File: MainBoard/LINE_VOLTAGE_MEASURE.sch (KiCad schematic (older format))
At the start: 18 parts

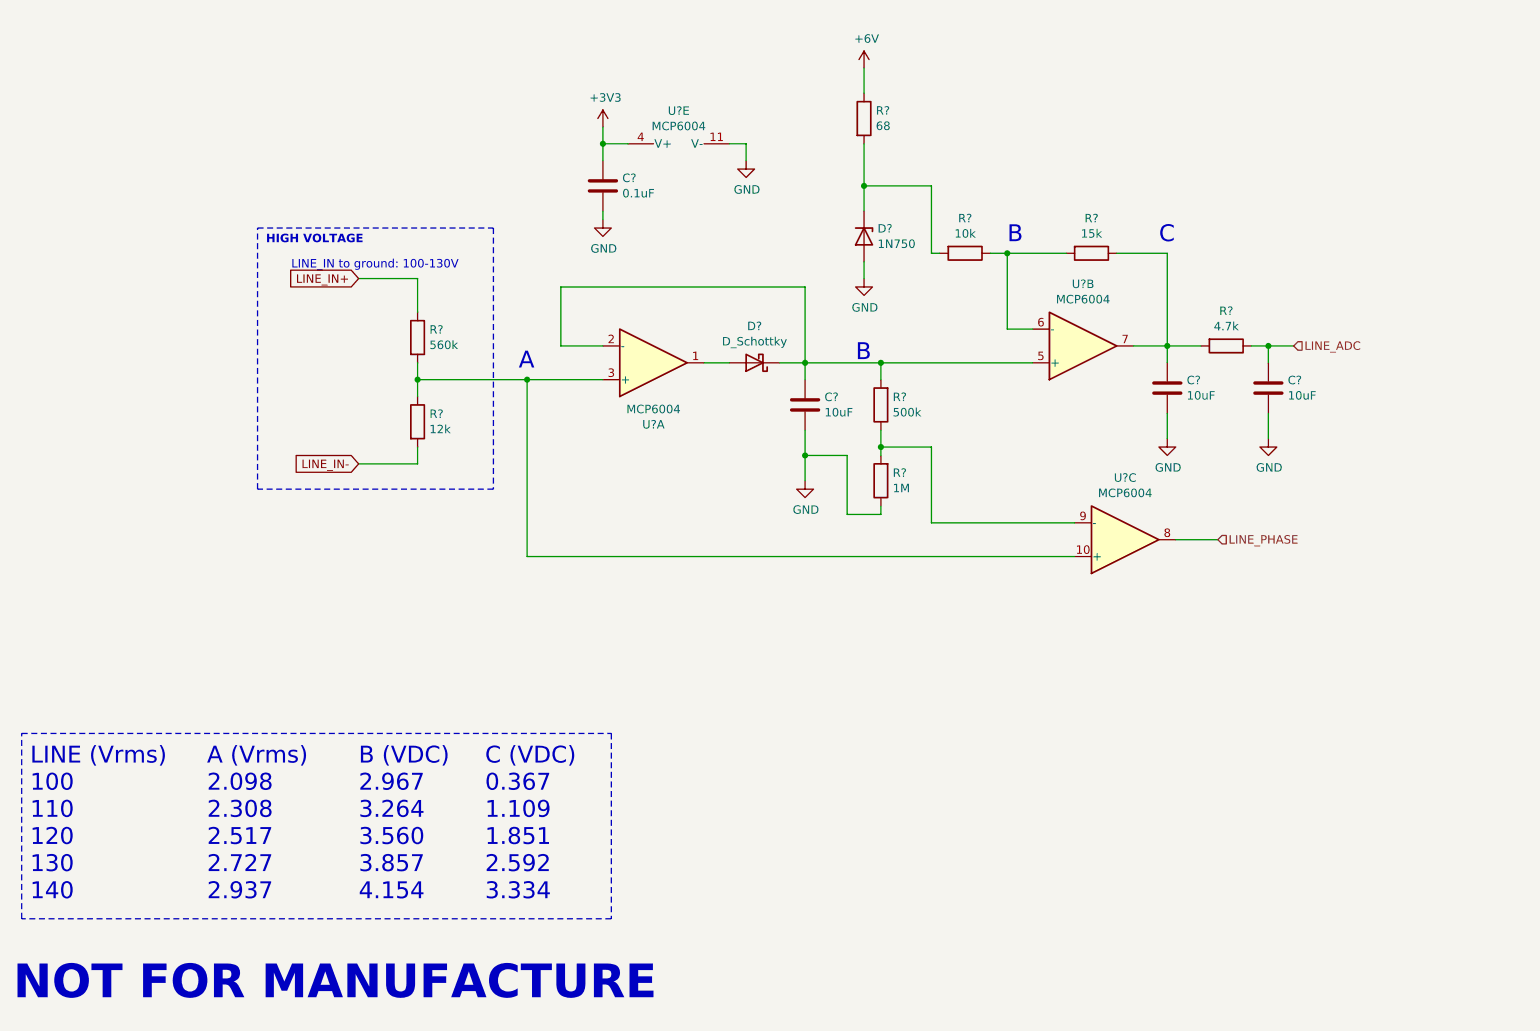
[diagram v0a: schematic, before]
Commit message: Layout Main Board
Layout main PCB
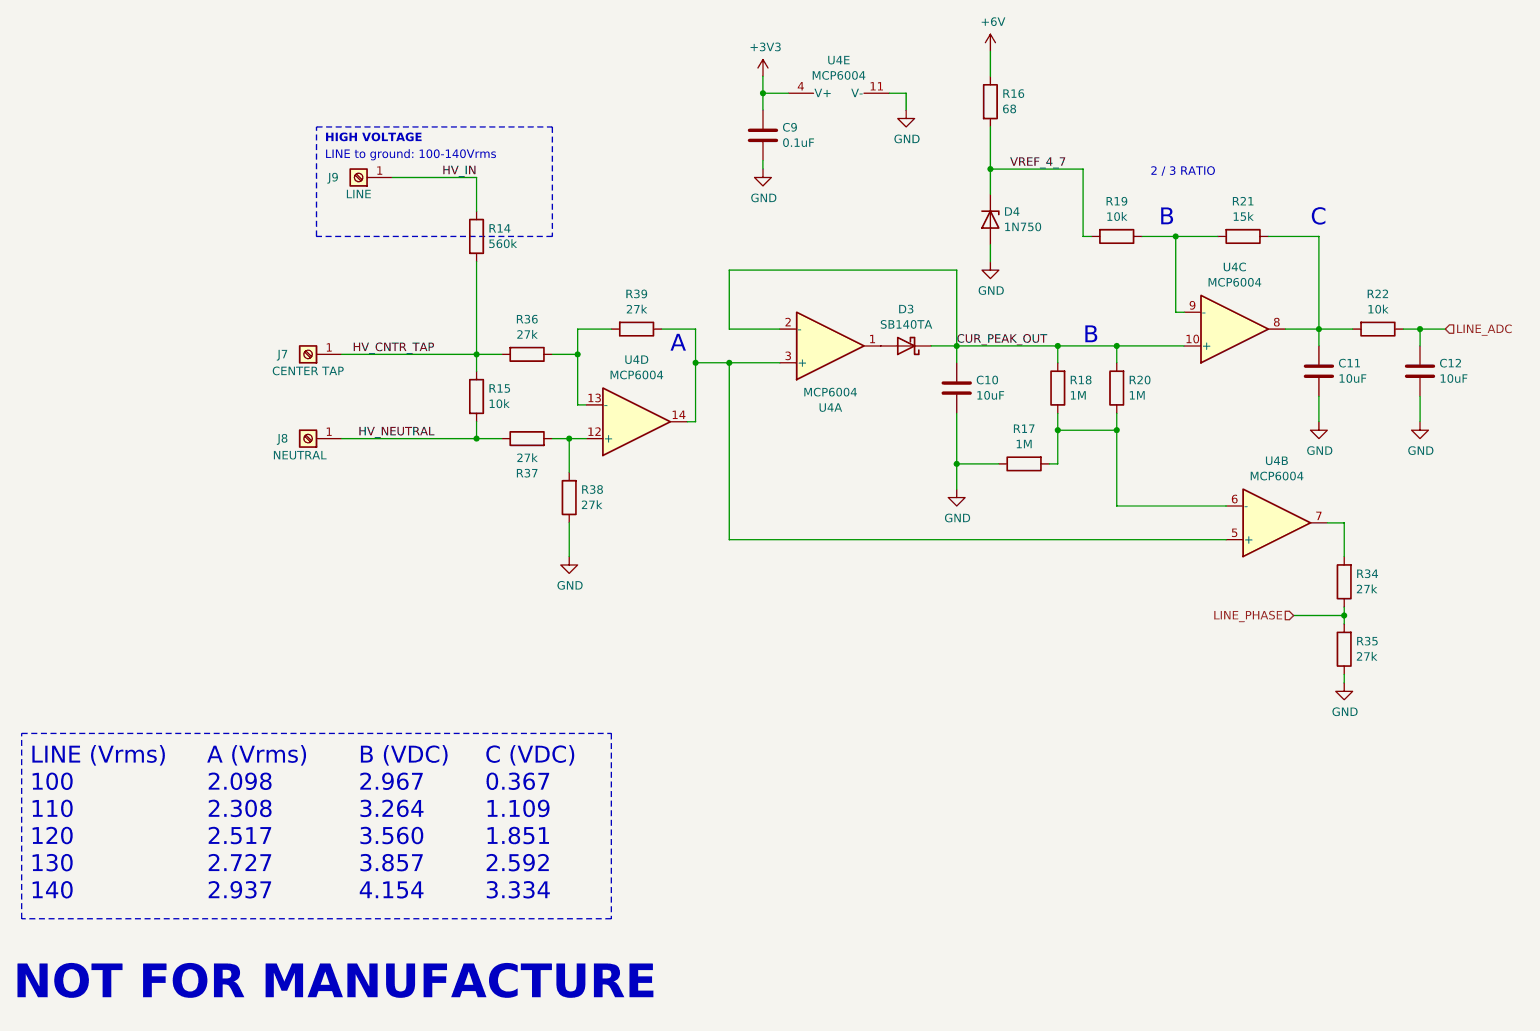
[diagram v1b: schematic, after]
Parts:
- removed R?: 4.7k, symbol Device:R
- removed R?: 1M, symbol Device:R
- removed R?: 500k, symbol Device:R
- added J7: CENTER TAP, Connector_PinHeader_2.54mm:PinHeader_1x01_P2.54mm_Vertical, symbol Connector:Screw_Terminal_01x01
- added J8: NEUTRAL, Connector_PinHeader_2.54mm:PinHeader_1x01_P2.54mm_Vertical, symbol Connector:Screw_Terminal_01x01
- added J9: LINE, Connector_PinHeader_2.54mm:PinHeader_1x01_P2.54mm_Vertical, symbol Connector:Screw_Terminal_01x01
- added R17, R18, R20: 1M, Resistor_THT:R_Axial_DIN0204_L3.6mm_D1.6mm_P7.62mm_Horizontal, symbol Device:R
- added R22: 10k, Resistor_THT:R_Axial_DIN0204_L3.6mm_D1.6mm_P7.62mm_Horizontal, symbol Device:R
- added R34, R35, R36, R37, R38, R39: 27k, Resistor_THT:R_Axial_DIN0204_L3.6mm_D1.6mm_P7.62mm_Horizontal, symbol Device:R
- added unit 4 of U4
- C10, C11, C12: renamed from C?; footprint (none) -> Capacitor_THT:CP_Radial_D5.0mm_P2.00mm; P/N (none) -> 732-8625-1-ND
- C9: renamed from C?; footprint (none) -> Capacitor_THT:C_Rect_L4.0mm_W2.5mm_P2.50mm
- D3: renamed from D?; value D_Schottky -> SB140TA; footprint (none) -> Diode_THT:D_DO-41_SOD81_P10.16mm_Horizontal; P/N (none) -> SB140TA
- D4: renamed from D?; footprint (none) -> Diode_THT:D_DO-35_SOD27_P10.16mm_Horizontal; P/N (none) -> 1514-1N750ABKPBFREE-ND
- R14: renamed from R?; footprint (none) -> Resistor_THT:R_Axial_DIN0207_L6.3mm_D2.5mm_P10.16mm_Horizontal
- R15: renamed from R?; value 12k -> 10k; footprint (none) -> Resistor_THT:R_Axial_DIN0204_L3.6mm_D1.6mm_P7.62mm_Horizontal
- R16, R21: renamed from R?; footprint (none) -> Resistor_THT:R_Axial_DIN0204_L3.6mm_D1.6mm_P7.62mm_Horizontal
- R19: renamed from R?; footprint Option in Mechatronics -> Resistor_THT:R_Axial_DIN0204_L3.6mm_D1.6mm_P7.62mm_Horizontal
- U4: renamed from U?; footprint (none) -> Package_DIP:DIP-14_W7.62mm_LongPads
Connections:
- net GND: now also R17.1, R35.1, R38.1
- net LINE_ADC: now also R22.1
- net LINE_PHASE: now also R34.1, R35.2; no longer U4.8
- net HV_CNTR_TAP: now reaches R14.2, R15.1
- net HV_CNTR_TAP: now also J7.1 (Pin_1), R36.2; no longer U4.10 (+), U4.3 (+)
- net CUR_PEAK_OUT: now reaches C10.1, D3.1 (K), U4.2 (-)
- net CUR_PEAK_OUT: now also U4.10 (+), R18.2, R20.2; no longer U4.5 (+)
- net at C11.1, R21.1: now also U4.8, R22.2; no longer U4.7
- net at R19.1, R21.2: now also U4.9 (-); no longer U4.6 (-)
- net VREF_4_7: now reaches D4.1 (K), R16.2, R19.2
- net LINE_IN+ renamed HV_IN
- net HV_IN: now also J9.1 (Pin_1)
- net LINE_IN- renamed HV_NEUTRAL
- net HV_NEUTRAL: now also J8.1 (Pin_1), R37.1
- new net: R39.1, U4.14, U4.3 (+), U4.5 (+)
- new net: R17.2, R18.1, R20.1, U4.6 (-)
- new net: R34.2, U4.7
- new net: R37.2, R38.2, U4.12 (+)
- new net: R36.1, R39.2, U4.13 (-)
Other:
- note added: "2 / 3 RATIO"
- note added: "LINE to ground: 100-140Vrms\n"
- note removed: "LINE_IN to ground: 100-130V\n"
- moved on the sheet: C10, C11, C12, C9, D3, D4, R14, R15, R16, R19, R21, U4A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
